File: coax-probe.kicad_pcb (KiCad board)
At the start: 2 copper layers, 27.8 x 34 mm, 33 parts, among them J1 Conn_01x02, J2 SMA, J3 Conn_01x02, J4 Conn_01x03, J5 SMA, J6 Conn_01x02, U1 OPA690, U2 INA128, U3 OPA690, U4 CJ431, U5 ICL7660

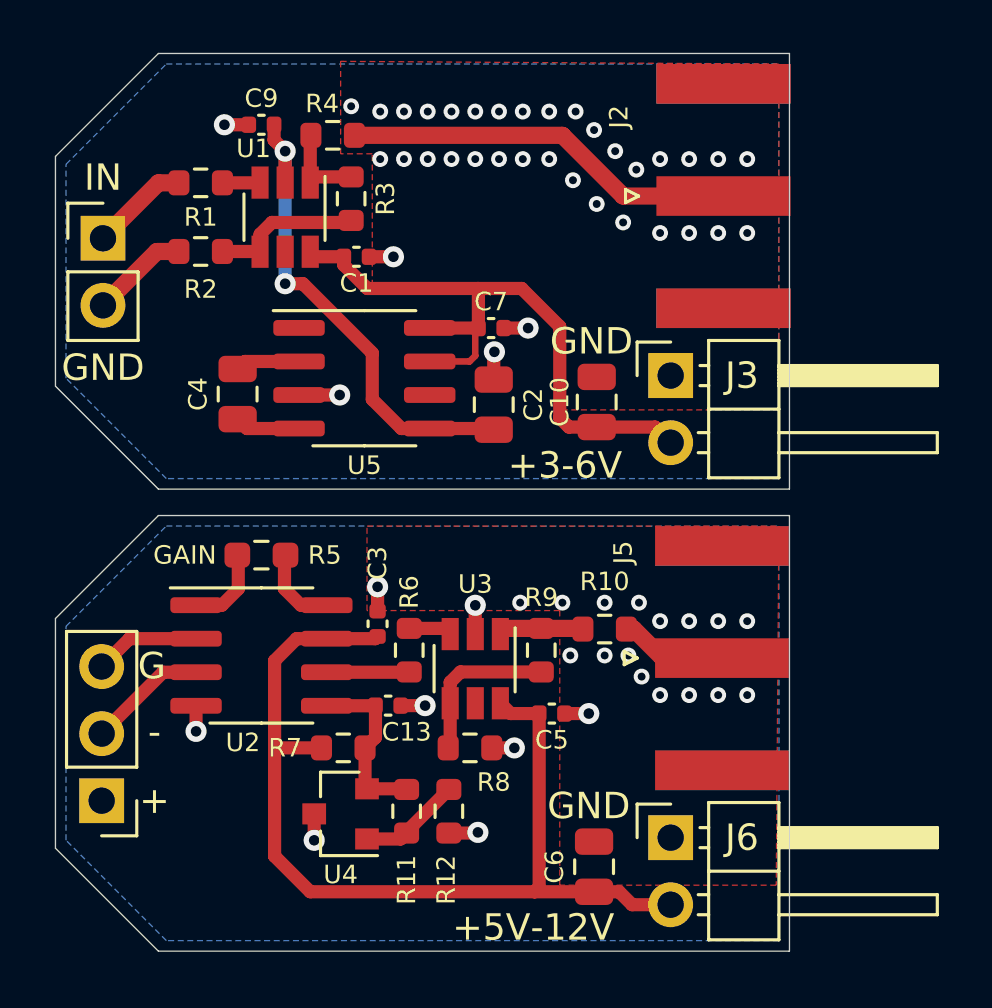
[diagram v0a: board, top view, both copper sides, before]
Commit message: Tweak zones.
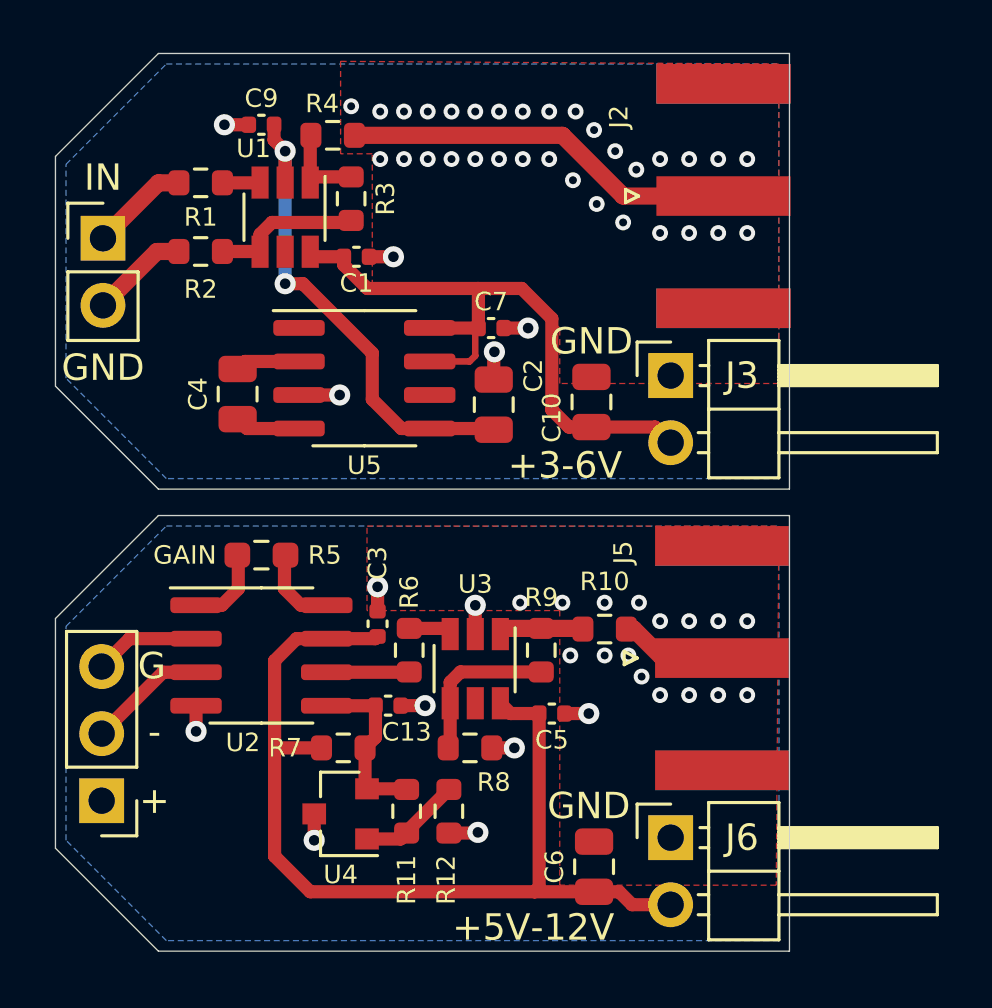
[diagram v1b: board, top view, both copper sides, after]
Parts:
- moved C10 0.20 mm to (177.5, 66.7)
